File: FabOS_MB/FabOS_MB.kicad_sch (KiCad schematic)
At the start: 3 parts, among them U1 STM32F407VETx

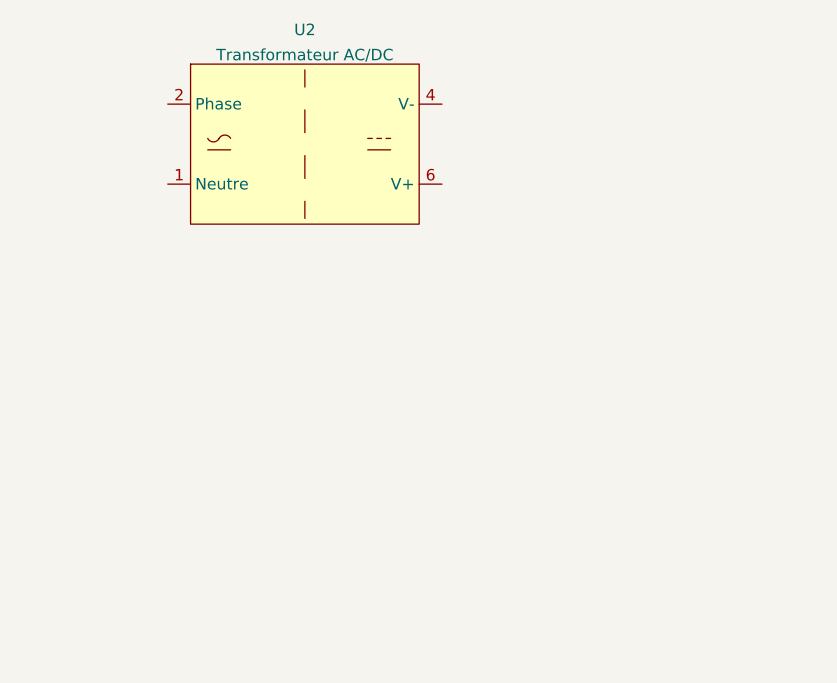
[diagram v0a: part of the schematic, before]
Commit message: Mise à jour empreintes
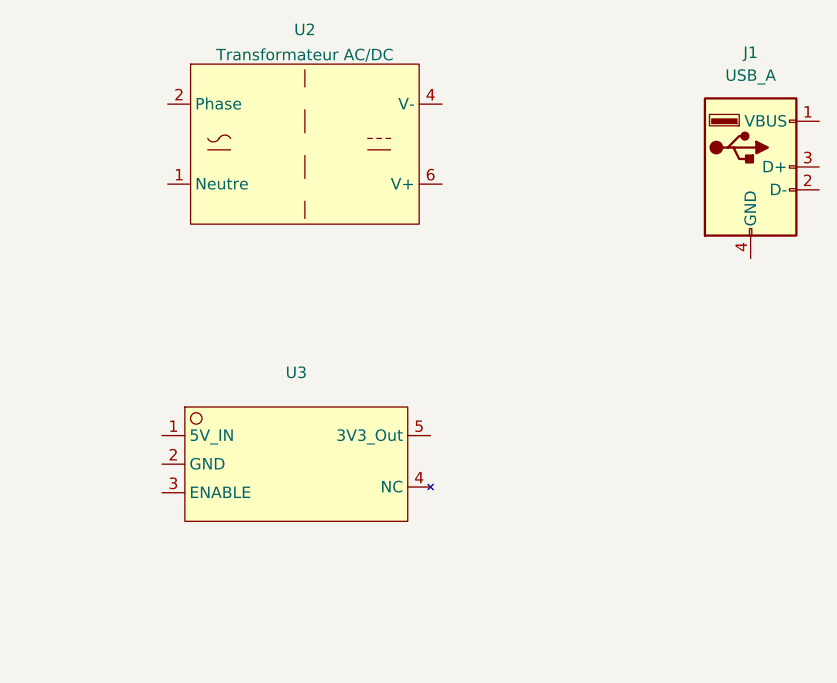
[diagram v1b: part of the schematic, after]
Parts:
- added J1: USB_A, Librairie_MB:USB_A_Femelle, symbol Connector:USB_A
- added U3: ~, Librairie_MB:Regulateur_tension_5V_3V3, symbol Librairie_MB:Regulateur_tension
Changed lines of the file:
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@@
+		)
+	)
+	(symbol
+		(lib_id "Connector:USB_A")
+		(at 255.27 38.1 0)
+		(unit 1)
+		(exclude_from_sim no)
+		(in_bom yes)
+		(on_board yes)
+		(dnp no)
+		(fields_autoplaced yes)
+		(property "Reference" "J1"
+			(at 255.27 25.4 0)
+			(effects
+				(font
+					(size 1.27 1.27)
+				)
+			)
+		)
+		(property "Value" "USB_A"
+			(at 255.27 27.94 0)
+			(effects
+				(font
+					(size 1.27 1.27)
+				)
+			)
+		)
+		(property "Footprint" "Librairie_MB:USB_A_Femelle"
+			(at 259.08 39.37 0)
+			(effects
+				(font
+					(size 1.27 1.27)
+				)
+				(hide yes)
+			)
+		)
+		(property "Datasheet" "https://www.lcsc.com/datasheet/lcsc_datasheet_2103011233_Jing-Extension-of-the-Electronic-Co--908-371A1011D10100_C42576.pdf"
+			(at 259.08 39.37 0)
+			(effects
+				(font
+					(size 1.27 1.27)
+				)
+				(hide yes)
+			)
+		)
+		(property "Description" "USB Type A connector"
+			(at 255.27 38.1 0)
+			(effects
+				(font
+					(size 1.27 1.27)
+				)
+				(hide yes)
+			)
+		)
+		(property "MPN" "  908-371A1011D10100"
+			(at 255.27 38.1 0)
+			(effects
+				(font
+					(size 1.27 1.27)
+				)
+				(hide yes)
+			)
+		)
+		(property "LCSC" "  C42576"
+			(at 255.27 38.1 0)
+			(effects
+				(font
+					(size 1.27 1.27)
+				)
+				(hide yes)
+			)
+		)
+		(pin "2"
+		)
+		(pin "4"
+		)
+		(pin "1"
+		)
+		(pin "3"
+		)
+		(instances
+			(project ""
+				(path "/09377d5d-727f-4ff4-92c8-7a0483d23f1e"
+					(reference "J1")
+					(unit 1)
+				)
+			)
+		)
+	)
+	(symbol
+		(lib_id "Librairie_MB:Regulateur_tension")
+		(at 204.47 71.12 0)
+		(unit 1)
+		(exclude_from_sim no)
+		(in_bom yes)
+		(on_board yes)
+		(dnp no)
+		(fields_autoplaced yes)
+		(property "Reference" "U3"
+			(at 204.7875 60.96 0)
+			(effects
+				(font
+					(size 1.27 1.27)
+				)
+			)
+		)
+		(property "Value" "~"
+			(at 204.7875 63.5 0)
+			(effects
+				(font
+					(size 1.27 1.27)
+				)
+			)
+		)
+		(property "Footprint" "Librairie_MB:Regulateur_tension_5V_3V3"
+			(at 203.835 81.28 0)
+			(effects
+				(font
+					(size 1.27 1.27)
+				)
+				(hide yes)
+			)
+		)
+		(property "Datasheet" "https://www.lcsc.com/datasheet/lcsc_datasheet_2304140030_Seaward-Elec-SE5218ALG-LF_C118233.pdf"
+			(at 207.645 53.34 0)
+			(effects
+				(font
+					(size 1.27 1.27)
+				)
+				(hide yes)
+			)
+		)
+		(property "Description" ""
+			(at 204.47 71.12 0)
+			(effects
+				(font
+					(size 1.27 1.27)
+				)
+				(hide yes)
+			)
+		)
+		(property "MPN" "  SE5218ALG-LF"
+			(at 204.47 56.515 0)
+			(effects
+				(font
+					(size 1.27 1.27)
+				)
+				(hide yes)
+			)
+		)
+		(property "LCSC" "C118233"
+			(at 205.74 59.055 0)
+			(effects
+				(font
+					(size 1.27 1.27)
+				)
+				(hide yes)
+			)
+		)
+		(pin "4"
+		)
+		(pin "1"
+		)
+		(pin "2"
+		)
+		(pin "3"
+		)
+		(pin "5"
+		)
+		(instances
+			(project ""
+				(path "/09377d5d-727f-4ff4-92c8-7a0483d23f1e"
+					(reference "U3")
+					(unit 1)
+				)
+			)
 		)
 	)
